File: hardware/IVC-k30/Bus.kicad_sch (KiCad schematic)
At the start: 1 part, among them U17 VME64-P1-5R-NS

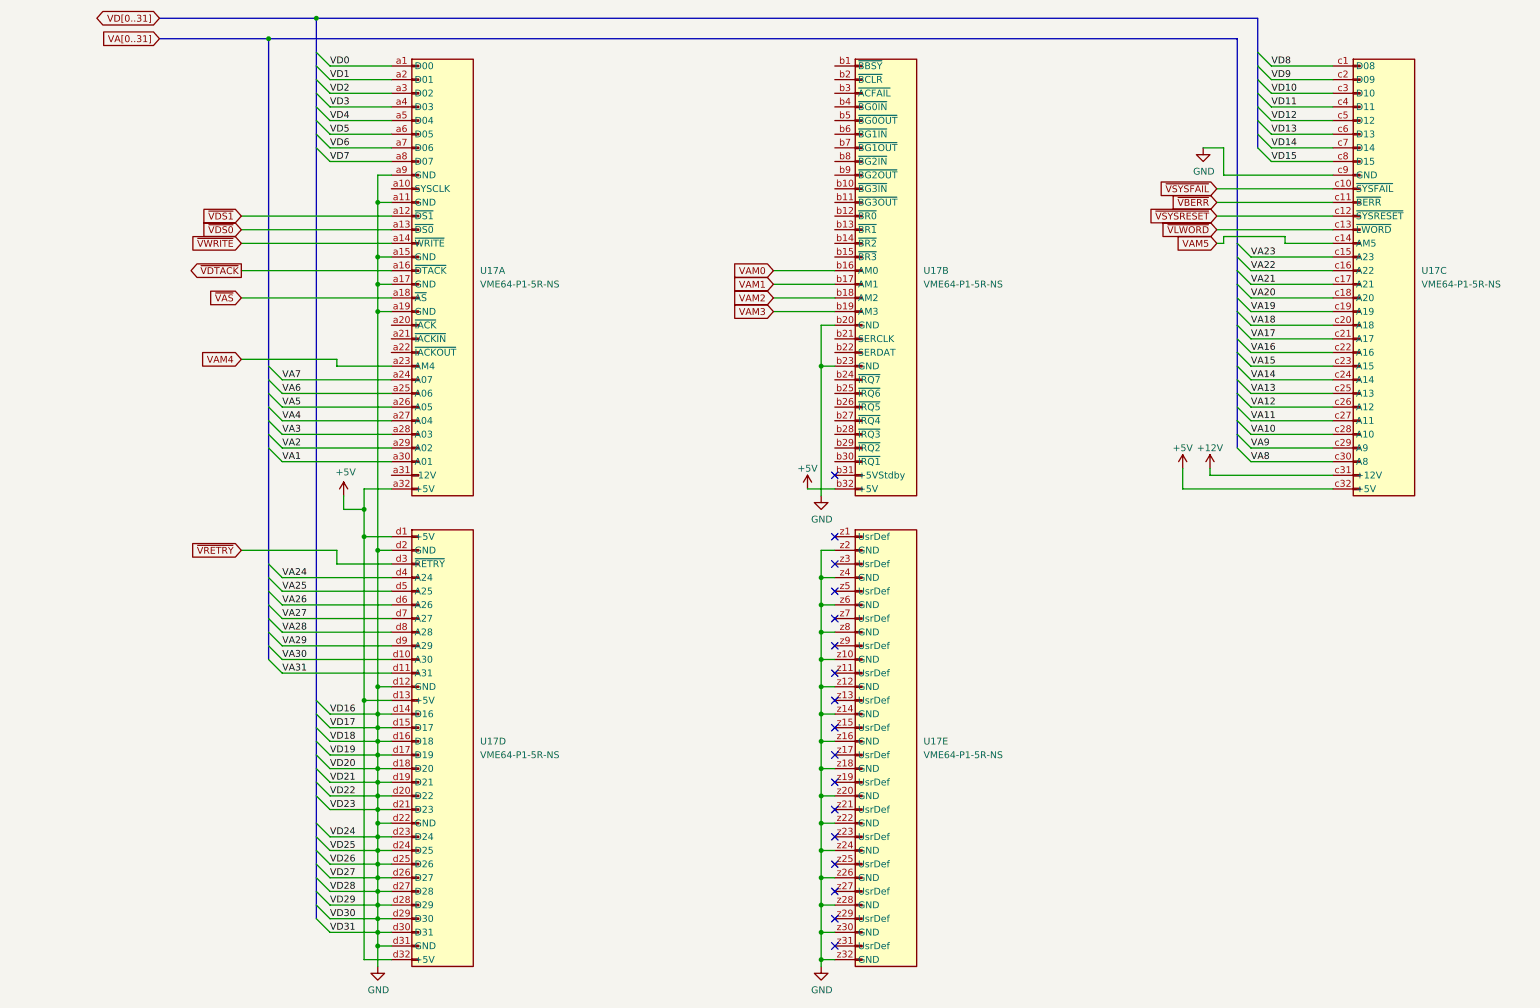
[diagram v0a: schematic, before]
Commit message: Committed changes to k30 board from Oct 9th 2023
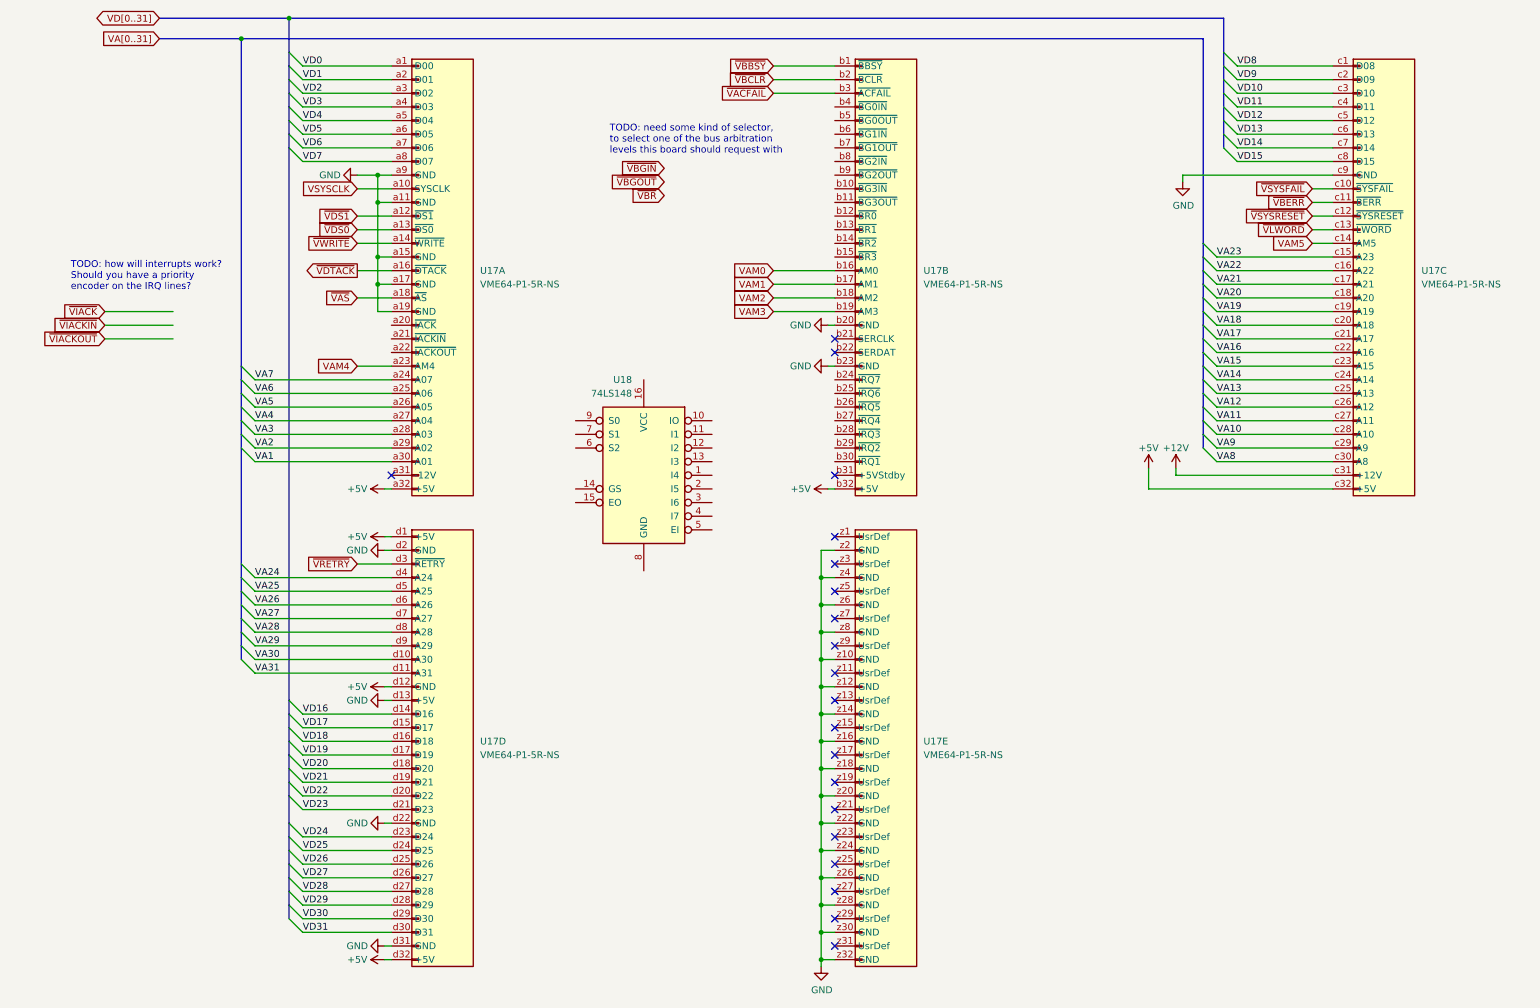
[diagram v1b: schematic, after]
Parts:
- added U18: 74LS148, symbol 74xx:74LS148
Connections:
- net +5V: now also U17.d12 (GND); no longer U17.d13 (+5V)
- net GND: now also U17.d13 (+5V); no longer U17.d12 (GND), U17.d14 (D16), U17.d15 (D17), U17.d16 (D18), U17.d17 (D19), U17.d18 (D20), U17.d19 (D21), U17.d20 (D22), U17.d21 (D23), U17.d23 (D24), U17.d24 (D25), U17.d25 (D26), U17.d26 (D27), U17.d27 (D28), U17.d28 (D29), U17.d29 (D30), U17.d30 (D31)
- net ~{VBBSY}: now reaches U17.b1 (~{BBSY})
- net ~{VBCLR}: now reaches U17.b2 (~{BCLR})
- net ~{VACFAIL}: now reaches U17.b3 (~{ACFAIL})
- net VSYSCLK: now reaches U17.a10 (SYSCLK)
- new net VD16: U17.d14 (D16)
- new net VD17: U17.d15 (D17)
- new net VD18: U17.d16 (D18)
- new net VD19: U17.d17 (D19)
- new net VD20: U17.d18 (D20)
- new net VD21: U17.d19 (D21)
- new net VD22: U17.d20 (D22)
- new net VD23: U17.d21 (D23)
- new net VD24: U17.d23 (D24)
- new net VD25: U17.d24 (D25)
- new net VD26: U17.d25 (D26)
- new net VD27: U17.d26 (D27)
- new net VD28: U17.d27 (D28)
- new net VD29: U17.d28 (D29)
- new net VD30: U17.d29 (D30)
- new net VD31: U17.d30 (D31)
- no-connect marks 17 -> 20
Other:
- note added: "TODO: how will interrupts work? Should you have a priority encoder on the IRQ lines?"
- note added: "TODO: need some kind of selector, to select one of the bus arbitration levels this board should request with"
